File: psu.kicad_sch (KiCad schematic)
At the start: 38 parts, among them J1 USB_B_Micro, J6 Screw_Terminal_01x02, J7 Barrel_Jack_MountingPin, Q1 FDS4435BZ, U1 NCP1117-3.3_SOT223, U6 AP64501SP-13

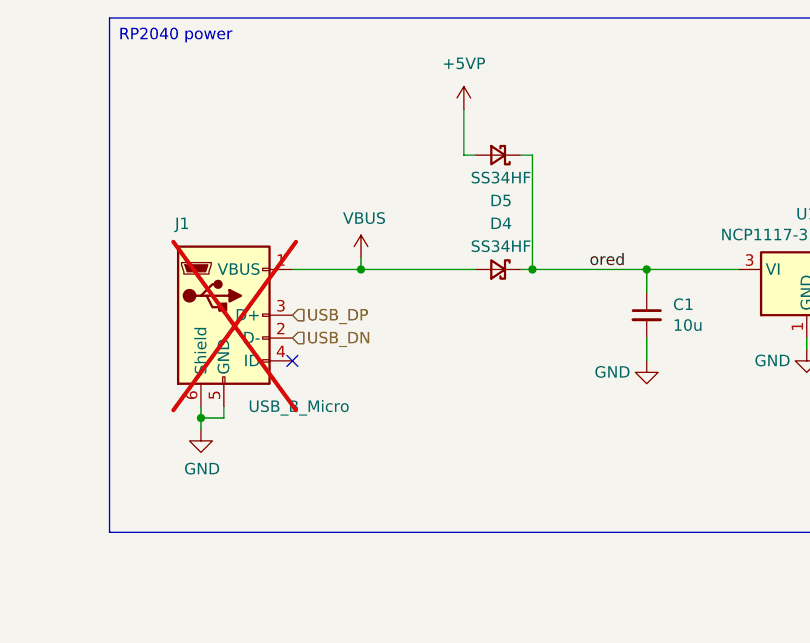
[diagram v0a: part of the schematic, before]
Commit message: First version of USB-Hub
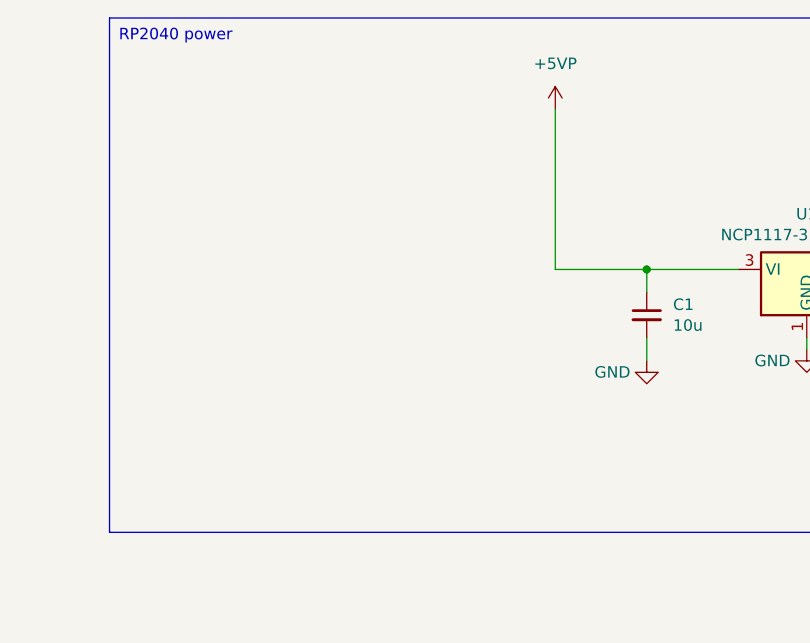
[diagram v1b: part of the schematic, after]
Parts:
- removed D4, D5: SS34HF, Diode_SMD:D_SMA, symbol Device:D_Schottky_Small
- removed J1: USB_B_Micro, Pedalboard Library:USB_Micro-B_Wuerth_614105150721_Vertical, symbol pedalboard:USB_B_Micro-Connector
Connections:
- net ored is gone; now on net +5VP: C1.1, U1.3 (VI)
- no-connect marks 2 -> 1

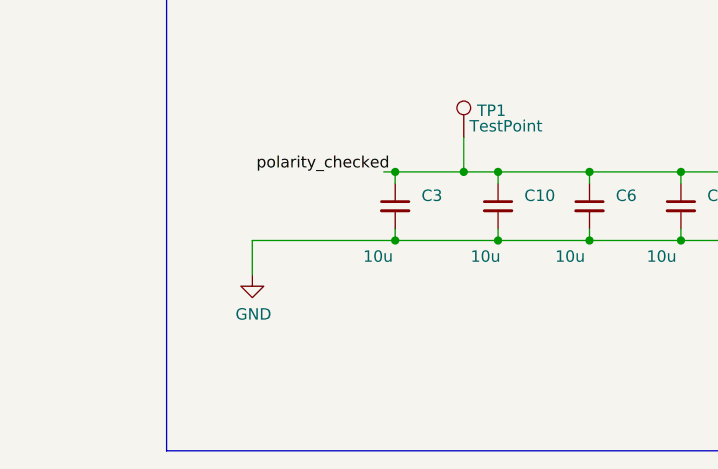
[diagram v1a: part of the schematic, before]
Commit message: Fix symbol warnings
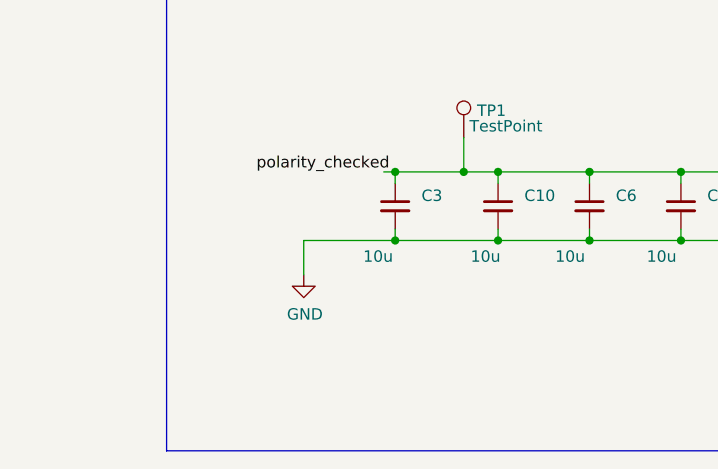
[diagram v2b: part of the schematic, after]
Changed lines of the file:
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@@
 	(wire
 		(pts
-			(xy 42.545 130.81) (xy 42.545 134.62)
+			(xy 48.26 130.81) (xy 48.26 134.62)
 		)
 		(stroke
@@
 	(wire
 		(pts
-			(xy 42.545 130.81) (xy 58.42 130.81)
+			(xy 48.26 130.81) (xy 58.42 130.81)
 		)
 		(stroke
@@
 			)
 		)
-		(property "Description" ""
+		(property "Description" "Power symbol creates a global label with name \"GND\" , ground"
 			(at 135.89 146.05 0)
 			(effects
@@
 			)
 		)
-		(property "Description" ""
+		(property "Description" "Power symbol creates a global label with name \"GND\" , ground"
 			(at 223.52 53.34 0)
 			(effects
@@
 			)
 		)
-		(property "Description" ""
+		(property "Description" "Power symbol creates a global label with name \"GND\" , ground"
 			(at 241.3 54.61 0)
 			(effects
@@
 	)
 	(symbol
-		(lib_name "GND_1")
 		(lib_id "power:GND")
 		(at 45.72 77.47 0)
@@
 			)
 		)
-		(property "Description" ""
+		(property "Description" "Power symbol creates a global label with name \"GND\" , ground"
 			(at 45.72 77.47 0)
 			(effects
@@
 			)
 		)
-		(property "Description" ""
+		(property "Description" "Power symbol creates a global label with name \"GND\" , ground"
 			(at 205.74 54.61 0)
 			(effects
@@
 			)
 		)
-		(property "Description" ""
+		(property "Description" "Power symbol creates a global label with name \"GND\" , ground"
 			(at 245.237 119.38 0)
 			(effects
@@
 			)
 		)
-		(property "Description" ""
+		(property "Description" "Power symbol creates a global label with name \"GND\" , ground"
 			(at 201.295 132.08 0)
 			(effects
@@
 			)
 		)
-		(property "Description" ""
+		(property "Description" "Power symbol creates a global label with name \"+5VP\""
 			(at 254.635 109.22 0)
 			(effects
@@
 	(symbol
 		(lib_id "power:GND")
-		(at 42.545 134.62 0)
+		(at 48.26 134.62 0)
 		(unit 1)
 		(exclude_from_sim no)
@@
 		(dnp no)
 		(property "Reference" "#PWR059"
-			(at 42.545 140.97 0)
+			(at 48.26 140.97 0)
 			(effects
 				(font
@@
 		)
 		(property "Value" "GND"
-			(at 42.672 139.0142 0)
+			(at 48.387 139.0142 0)
 			(effects
 				(font
@@
 		)
 		(property "Footprint" ""
-			(at 42.545 134.62 0)
+			(at 48.26 134.62 0)
 			(effects
 				(font
@@
 		)
 		(property "Datasheet" ""
-			(at 42.545 134.62 0)
+			(at 48.26 134.62 0)
 			(effects
 				(font
@@
 			)
 		)
-		(property "Description" ""
-			(at 42.545 134.62 0)
+		(property "Description" "Power symbol creates a global label with name \"GND\" , ground"
+			(at 48.26 134.62 0)
 			(effects
 				(font
@@
 			)
 		)
-		(property "Description" ""
+		(property "Description" "Power symbol creates a global label with name \"GND\" , ground"
 			(at 201.93 119.38 0)
 			(effects
@@
 			)
 		)
-		(property "Description" ""
+		(property "Description" "Power symbol creates a global label with name \"+3V3\""
 			(at 241.3 43.18 0)
 			(effects
@@
 			)
 		)
-		(property "Description" ""
+		(property "Description" "Power symbol creates a global label with name \"+5VP\""
 			(at 195.58 26.67 0)
 			(effects

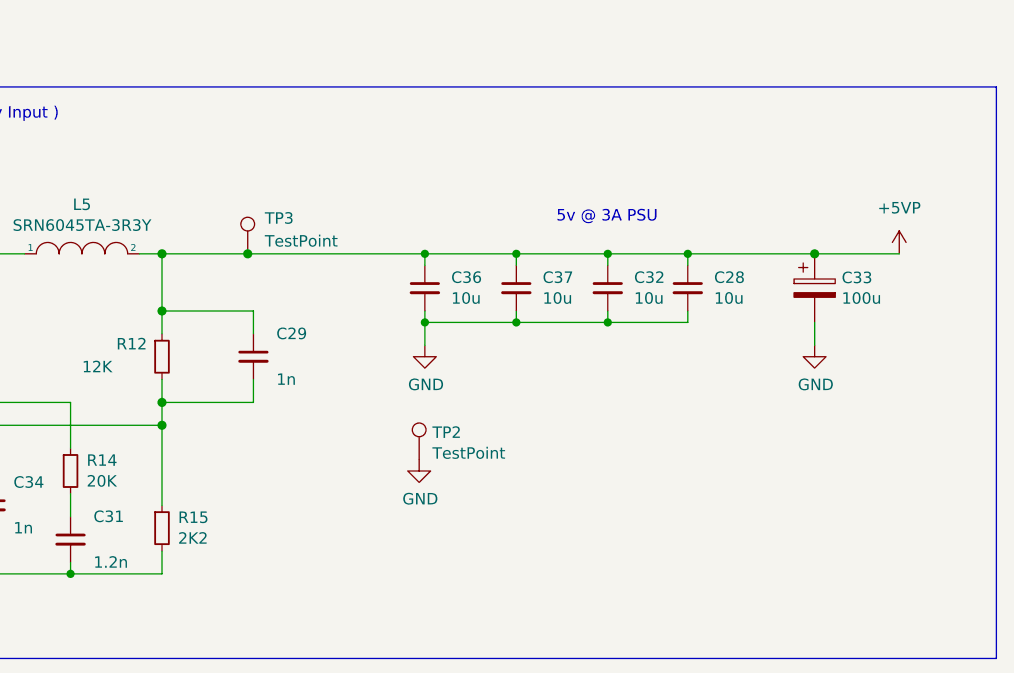
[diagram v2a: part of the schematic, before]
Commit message: Fix warngings
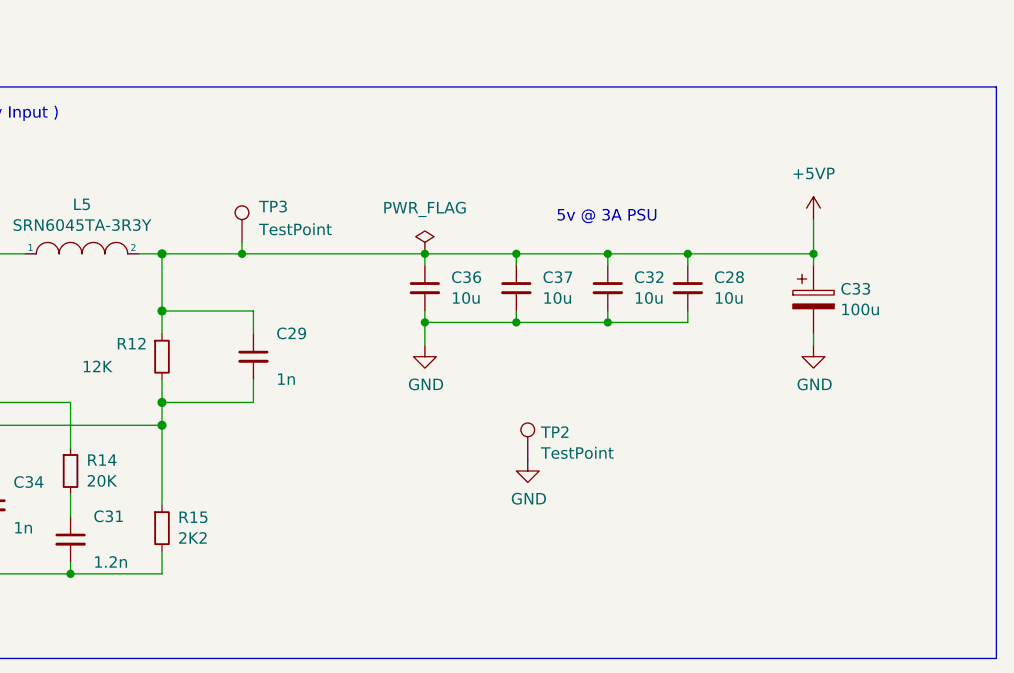
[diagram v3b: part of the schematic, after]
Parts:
- C33: symbol Device:CP -> Device:C_Polarized
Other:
- moved on the sheet: C33, TP2, TP3
